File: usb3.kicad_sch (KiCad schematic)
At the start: 44 parts, among them J4 USB3_A, J5 Conn_01x15_MountingPin, J6 USB_C_Receptacle_USB2.0_16P, Q1 2N7002, U10 TPD4E05U06QDQARQ1, U11 TPD4E05U06QDQARQ1, U5 AP22615A, U6 AP22615A, U7 TPD4E05U06QDQARQ1, U8 TPD4E05U06QDQARQ1, U9 TPD4E05U06QDQARQ1

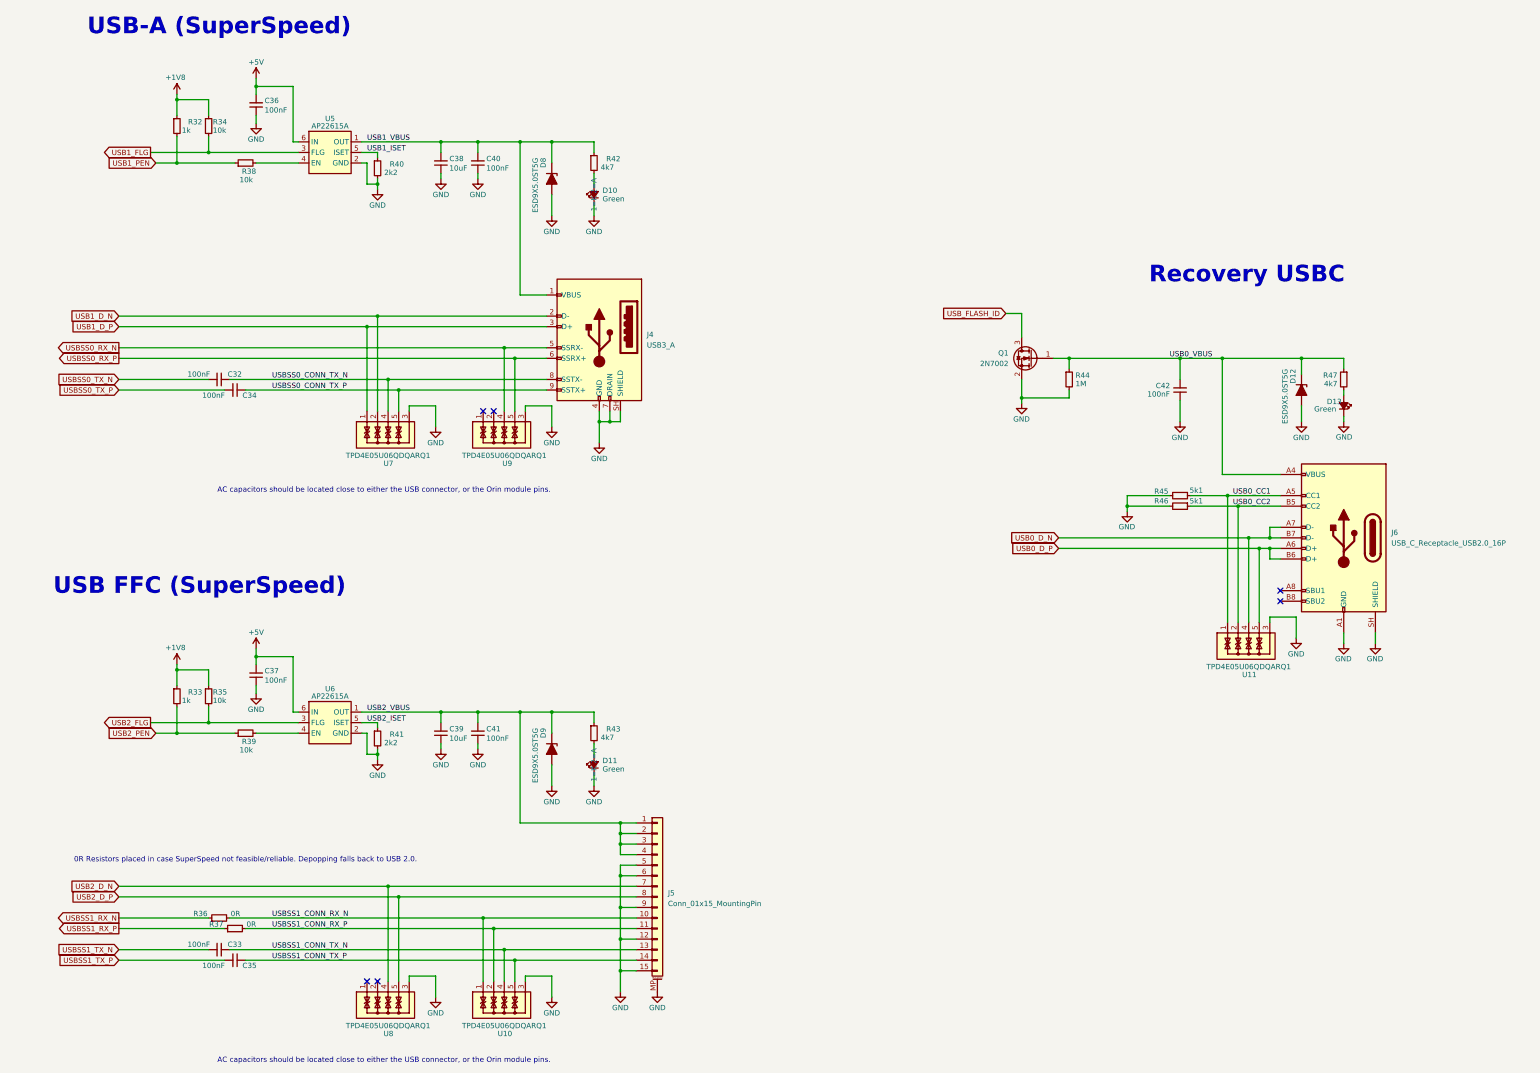
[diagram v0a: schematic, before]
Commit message: Final BOM changes, gerbers
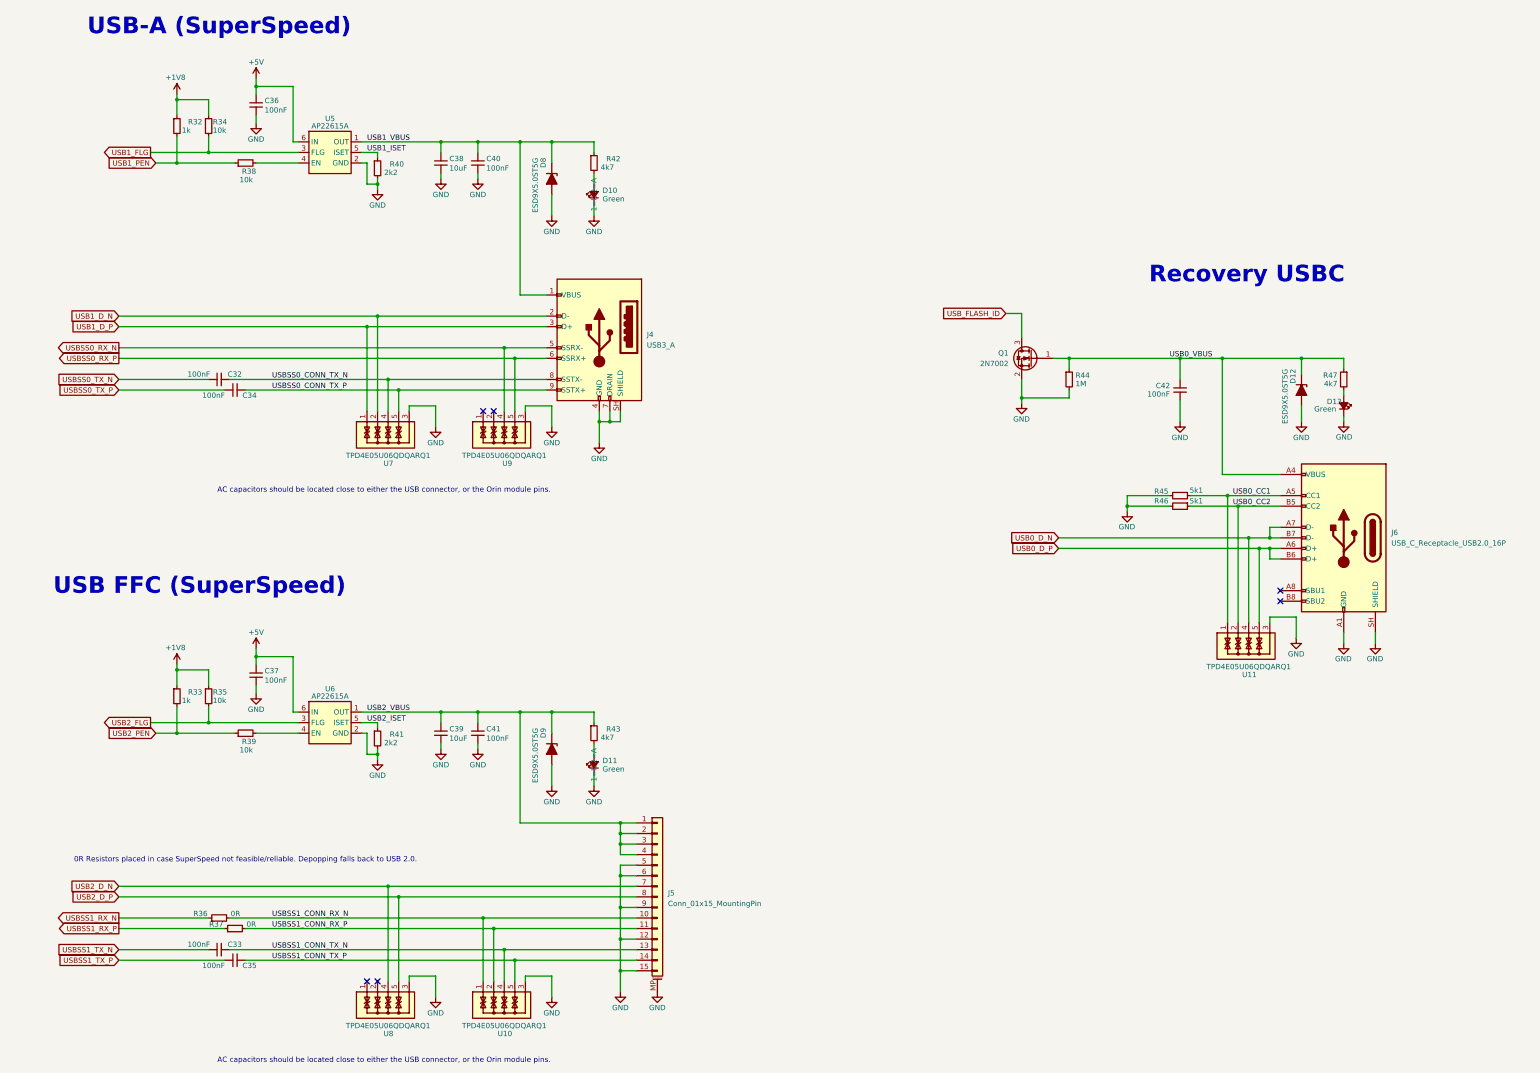
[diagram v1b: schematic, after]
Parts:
- C32, C33, C34, C35: LCSC (none) -> C307331
- C36, C37, C40, C41, C42: LCSC (none) -> C14663
- C38, C39: LCSC (none) -> C96446
- D10, D11, D13: LCSC (none) -> C12065
- D12, D8, D9: LCSC (none) -> C87910
- J4: LCSC (none) -> C473057
- J6: LCSC (none) -> C3020560
- Q1: LCSC (none) -> C8545
- R32, R33: LCSC (none) -> C21190
- R34, R35, R38, R39: LCSC (none) -> C25804
- R36, R37: LCSC (none) -> C17168
- R40, R41: LCSC (none) -> C4190
- R42, R43, R47: LCSC (none) -> C23162
- R44: LCSC (none) -> C22935
- R45, R46: LCSC (none) -> C23186
- U10, U11, U7, U8, U9: LCSC (none) -> C81353
- U5, U6: LCSC (none) -> C2680357
